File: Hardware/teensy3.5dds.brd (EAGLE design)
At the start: 95.8 x 84.1 mm, 97 parts, among them IC1 AD8034, IC2 AD8034, IC3 AD8034, IC5 AD8034, IC6 AD737KRZ-R7, IC7 AD8034, IC8 AD8034, J1 1776275-2, J2 1776275-2, Q1 10MHz, U1 TEENSY_3.5/3.6_BASIC, U2 ATMEGA32U4-AU, X1 1-227161-0

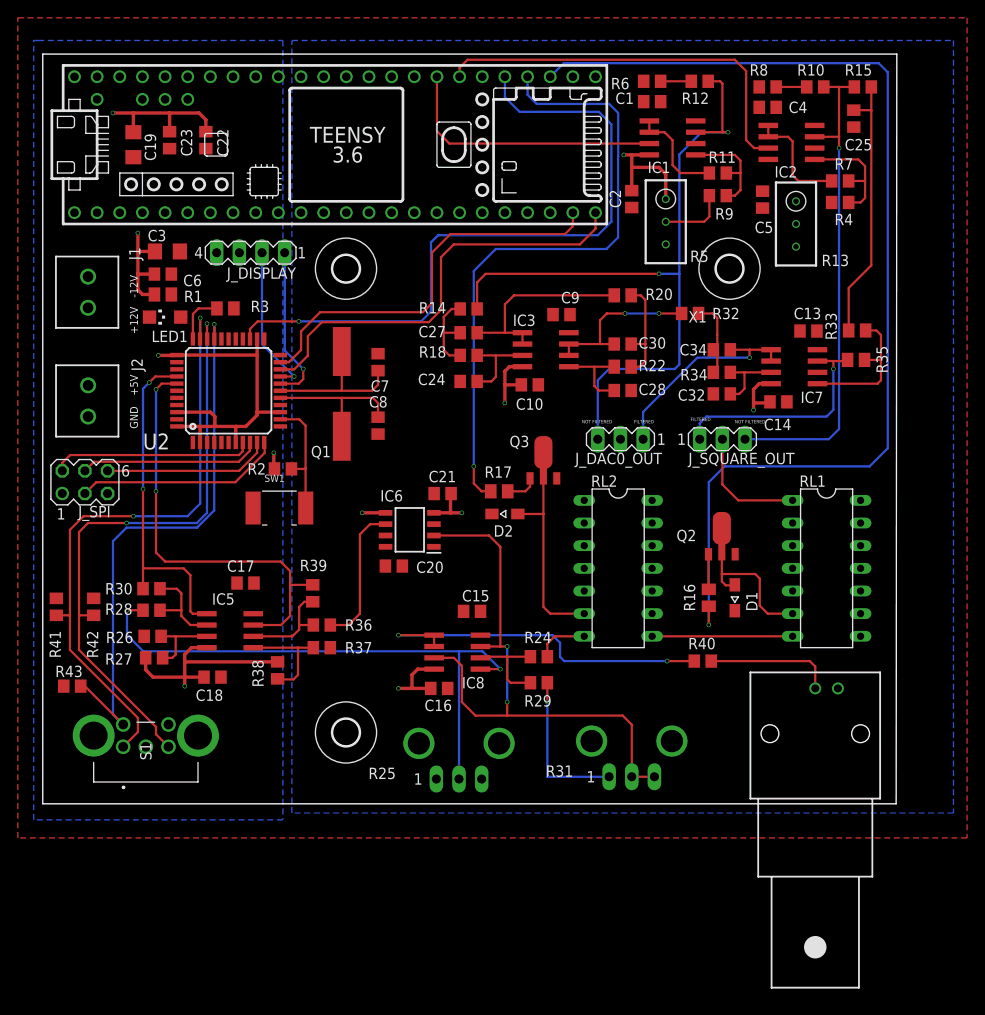
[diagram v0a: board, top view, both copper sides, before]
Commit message: fixes following the advice of people better than me at making PCBs
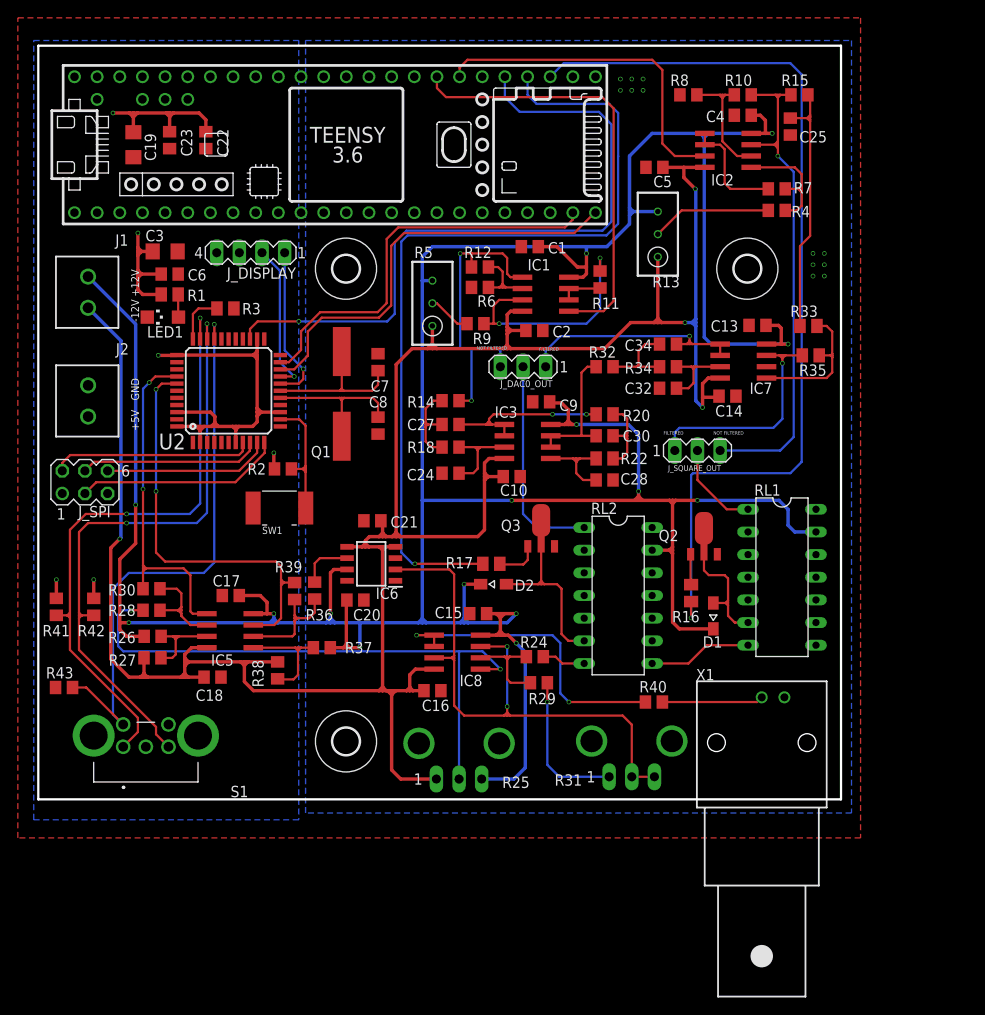
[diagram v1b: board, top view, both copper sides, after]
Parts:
- moved R12 32.3 mm to (49.0, 75.2), turned to 0 degrees
- moved R9 30.7 mm to (48.5, 68.8)
- moved R6 30.1 mm to (49.0, 72.9)
- moved R5 27.7 mm to (43.7, 71.1), turned to 0 degrees
- moved IC1 22.6 mm to (56.4, 72.1)
- moved C1 21.3 mm to (54.6, 77.5)
- moved C2 18.3 mm to (55.1, 68.1), turned to 180 degrees
- moved R11 17.8 mm to (62.5, 73.8), turned to 90 degrees
- moved R13 15.5 mm to (69.0, 78.9), turned to 0 degrees
- moved J_DAC0_OUT 13.6 mm to (53.8, 64.0)
- moved R20 13.5 mm to (63.0, 58.7)
- moved C5 12.7 mm to (68.6, 86.4), turned to 0 degrees
- moved R32 11.3 mm to (63.0, 64.0)
- moved R18 10.5 mm to (45.7, 55.0)
- moved C10 10.5 mm to (52.6, 51.7)
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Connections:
- removed net V-1: R13.1
- net DAC0: now also IC1.5; no longer IC1.3
- net DAC0_OFFSET: now also IC1.1; no longer IC1.7
- net N$21: now also IC1.2; no longer IC1.6
- net N$23: now also IC1.6, IC1.7; no longer IC1.1, IC1.2
- net N$26: now also IC1.3; no longer IC1.5
- net V-: now also R13.1
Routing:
- net V+: track 0.00 -> 409.1 mm, vias 0 -> 15
- net V-: track 68.7 -> 294.1 mm, vias 7 -> 4
- net DAC0_OFFSET: track 83.6 -> 35.0 mm
- net DAC0_SEL: track 70.8 -> 95.1 mm
- net DAC0_OUT: track 0.00 -> 24.0 mm
- net DAC0: track 30.5 -> 49.1 mm
- net SQUARE_SEL: track 120.8 -> 103.6 mm
- net +5V: track 71.3 -> 87.8 mm, vias 4 -> 6
- net N$26: track 12.0 -> 26.5 mm, vias 0 -> 2
- net N$20: track 0.00 -> 13.5 mm
- net N$24: track 3.43 -> 14.9 mm
- net N$14: track 16.1 -> 5.98 mm
- net N$23: track 11.5 -> 4.79 mm
- net SQUARE: track 44.6 -> 38.2 mm
- net N$19: track 40.6 -> 35.3 mm
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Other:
- board size 95.8 x 84.1 mm -> 90 x 84.5 mm

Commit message: board v1.0
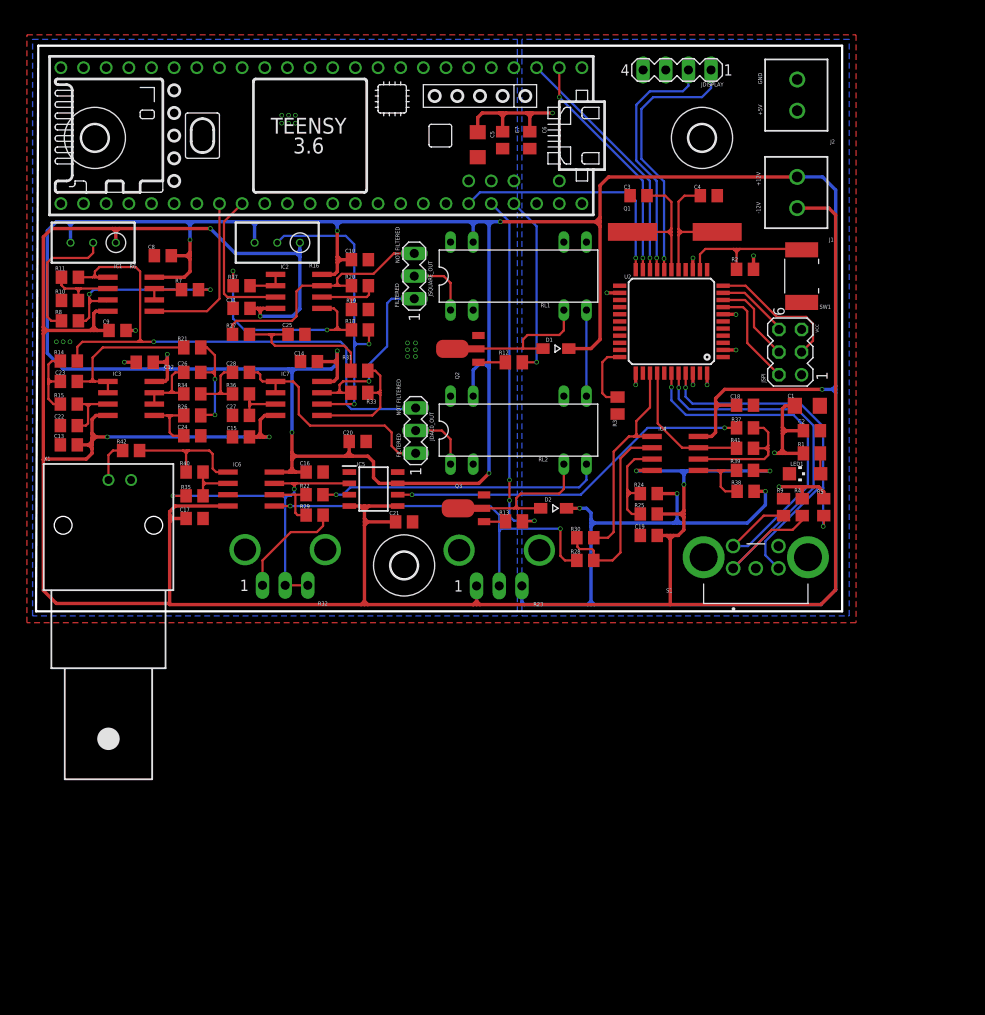
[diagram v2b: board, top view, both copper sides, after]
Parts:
- removed C30, C34: 100p, rcl:C0805
- removed C32: 10p, rcl:C0805
- removed IC8: AD8034, linear:SO08
- removed J_DAC0_OUT, J_SQUARE_OUT: (no value), con-lstb:MA03-1
- removed J_DISPLAY: (no value), con-lstb:MA04-1
- removed J_SPI: (no value), con-lstb:MA03-2
- removed R43: (no value), rcl:R0805
- removed U$5: (no value), holes:3,0
- added C11, C12: 100n, rcl:C0805
- added C26: 100p, rcl:C0805
- added IC4: AD8034, linear:SO08
- added JDAC0_OUT, JSQUARE_OUT: (no value), con-lstb:MA03-1
- added JDISPLAY: (no value), con-lstb:MA04-1
- added JSPI: (no value), con-lstb:MA03-2
- added R19: 1k, rcl:R0805
- added R21: 787, rcl:M0805
- added R23: 10k, Potentiometer_vertical:MA03-1
- added U$1: (no value), holes:3,0
- C1: value 100n -> 1u; device rcl:C0805 -> rcl:C1206
- C19: device rcl:C1206 -> rcl:C0805
- C22: value 100n -> 10p
- C23: value 1u -> 150p
- C25: value (none) -> 1p
- C27: value 100p -> 10p
- C28: value 10p -> 100p
- C3: value 1u -> 22p; device rcl:C1206 -> rcl:C0805
- C4: value 100n -> 22p
- C5: device rcl:C0805 -> rcl:C1206
- C7: value 22p -> 1u
- C8: value 22p -> 100n
- IC5: value AD8034 -> AD737KRZ-R7; device linear:SO08 -> AD737KRZ-R7:SOIC127P600X175-8N
- IC6: value AD737KRZ-R7 -> AD8034; device AD737KRZ-R7:SOIC127P600X175-8N -> linear:SO08
- Q1: value 10MHz -> 16MHz
- R12: value 1k -> 500; device rcl:R0805 -> rcl:M0805
- R13: value 100k -> 500; device rcl:RTRIM3296W -> rcl:M0805
- R15: value (none) -> 2.74k
- R16: value (none) -> 100k; device rcl:M0805 -> rcl:RTRIM3296W
- R17: value (none) -> 1k; device rcl:M0805 -> rcl:R0805
- R18: value 2.74k -> 1k
- R20: value 787 -> 1k; device rcl:M0805 -> rcl:R0805
- R22: value 14.3k -> 1k; device rcl:M0805 -> rcl:R0805
- R25: value 10k -> 1.5k; device Potentiometer_vertical:MA03-1 -> rcl:R0805
- R26: value (none) -> 14.3k; device rcl:R0805 -> rcl:M0805
- R27, R42: value (none) -> 50
- R28, R37: value (none) -> 5k
- R30, R41: value (none) -> 1k
- R31: value 10k -> 2k; device Potentiometer_vertical:MA03-1 -> rcl:M0805
- R32: value 562 -> 10k; device rcl:R0805 -> Potentiometer_vertical:MA03-1
- R33: value 243 -> 10k
- R34: value 20k -> 562
- R35: value 1.78k -> (none); device rcl:M0805 -> rcl:R0805
- R36: value (none) -> 20k
- R38: value (none) -> 10k
- R39: value (none) -> 14.3k
- R4, R9: value 1k -> 10k
- R40: value 50 -> (none)
- R5: value 100k -> 10k; device rcl:RTRIM3296W -> rcl:R0805
- R6: value 1k -> 100k; device rcl:R0805 -> rcl:RTRIM3296W
- RL1, RL2: value PRME_15005SOCKET -> PRME_15005NOSOCKET; device prme15005:DIL14_SOCKET -> prme15005:DIL14
- moved R15 89.0 mm to (2.92, 59.8), turned to 0 degrees
- moved J2 86.6 mm to (84.6, 92.7)
- moved J1 80.3 mm to (84.6, 81.8)
- moved R41 79.2 mm to (78.7, 54.9), turned to 180 degrees
- moved R10 78.9 mm to (3.05, 71.4)
- moved C13 78.4 mm to (2.92, 55.2), turned to 0 degrees
- moved X1 77.2 mm to (7.37, 46.2)
- moved R1 74.2 mm to (86.2, 54.3)
- moved LED1 74.1 mm to (85.5, 52.0)
- moved R8 73.8 mm to (3.05, 69.2), turned to 0 degrees
- moved C19 72.5 mm to (67.9, 45.1), turned to 0 degrees
- moved S1 71.3 mm to (79.9, 40.4)
- moved R35 70.9 mm to (17.0, 49.5), turned to 0 degrees
- moved C18 67.0 mm to (78.7, 59.7), turned to 0 degrees
- moved R7 66.7 mm to (16.5, 72.6)
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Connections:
- removed net N$20: R13.2, R4.1
- new net N$36: IC6.2, R35.2, R40.1
- new net N$37: IC7.6, R16.2, R18.1
- net +5V: now also C1.1, C2.1, C5.1, C7.1, JDISPLAY.3, JSPI.5, R4.1, R5.1; no longer C19.1, C22.1, C23.1, C3.1, J_DISPLAY.3, J_SPI.5, R41.1, R42.1
- net AMPL_MEASURE: now also IC4.7, R41.2, U2.37; no longer IC5.7, R39.2, U2.38
- net DAC0_FILTERED: now also C28.1, JDAC0_OUT.1; no longer C34.1, J_DAC0_OUT.1
- net DAC0_OFFSET: now also JDAC0_OUT.3, R11.1; no longer J_DAC0_OUT.3, R12.1
- net DAC0_OUT: now also JDAC0_OUT.2; no longer J_DAC0_OUT.2
- net DAC0_SEL: now also R13.1, U1.22/A8; no longer R17.1, U1.36/A17
- net GND: now also C10.2, C11.1, C12.2, C13.1, C14.2, C15.1, C16.2, C17.1, C18.2, C19.1, C2.2, C22.1, C27.1, C3.1, C4.1, C5.2, C7.2, C8.2, C9.1, IC5.3, IC5.8, JDISPLAY.4, JSPI.1, R10.2, R19.2, R9.1; no longer C10.1, C13.2, C14.1, C15.2, C16.1, C17.2, C18.1, C19.2, C2.1, C22.2, C23.2, C28.1, C3.2, C32.1, C4.2, C5.1, C7.1, C8.1, C9.2, IC6.8, IC7.6, J_DISPLAY.4, J_SPI.1, R43.1, R6.2, R8.2
- net INTERRUPT: now also U1.21/A7, U2.22; no longer U1.37/A18, U2.25
- net MISO: now also JSPI.3; no longer J_SPI.3
- net MOSI: now also JSPI.6; no longer J_SPI.6
- net N$1: now also R31.2, R33.1; no longer R33.2, R35.1
- net N$10: now also R22.1; no longer R24.1
- net N$11: now also IC4.2; no longer IC5.2
- net N$13: now also IC4.3, R24.1, R25.2; no longer IC5.3, R26.1, R27.2
- net N$14: now also IC5.6, R37.1; no longer IC6.6, R36.1
- net N$15: now also R32.1; no longer R31.1
- net N$16: now also IC4.6, R37.2, R41.1; no longer IC5.6, R36.2, R39.1
- net N$17: now also R12.2; no longer R16.2
- net N$18: now also R13.2; no longer R17.2
- net N$19: now also IC6.1, R40.2, R42.1; no longer IC8.1, IC8.2, R40.1
- net N$21: now also R10.1, R11.2; no longer R12.2, R6.1
- net N$22: now also IC4.5, R38.2, R39.1; no longer IC5.5, R37.2, R38.1
- net N$23: now also R7.1; no longer R11.1
- net N$24: now also R19.1, R20.2; no longer R10.2, R8.1
- net N$25: now also R4.2, U2.40; no longer R41.2, U2.32
- net N$26: now also R7.2, R8.2; no longer R11.2, R9.2
- net N$27: now also R17.1; no longer R7.1
- net N$28: now also R17.2, R18.2; no longer R4.2, R7.2
- net N$29: now also R9.2, U2.39; no longer R43.2, U2.30
- net N$3: now also IC6.5, R23.2; no longer IC8.5, R25.2
- net N$31: now also C3.2; no longer C7.2
- net N$34: now also R27.1, R31.1; no longer R15.1, R33.1
- net N$4: now also C4.2; no longer C8.2
- net N$5: now also IC6.6, R22.2; no longer IC8.6, R24.2
- net N$50: now also C23.2, R15.1; no longer C27.2, R18.1
- net N$53: now also C23.1, R21.1; no longer C27.1, R20.1
- net N$56: now also R6.2, R8.1; no longer R5.2, R9.1
- net N$58: now also C22.2, R15.2; no longer C24.2, R18.2
- net N$6: now also R42.2; no longer R40.2
- net N$61: now also C26.1, R21.2, R26.1; no longer C30.1, R20.2, R22.1
- net N$62: now also C26.2, R34.1; no longer C30.2, R32.1
- net N$63: now also C24.2, R26.2; no longer C28.2, R22.2
- net N$73: now also C28.2, R34.2, R36.1; no longer C34.2, R32.2, R34.1
- net N$75: now also C27.2, R36.2; no longer C32.2, R34.2
- net N$8: now also R5.2, U2.41; no longer R42.2, U2.31
- net N$9: now also IC5.2, IC6.7, R32.2, R32.3, R35.1; no longer IC6.2, IC8.3, IC8.7, R31.2, R31.3
- net OFF_MEASURE: now also IC4.1, U2.36; no longer IC5.1, U2.37
- net RX1: now also U1.1/TX; no longer U1.32/A13
- net SCK: now also JSPI.4; no longer J_SPI.4
- net SCL: now also JDISPLAY.1; no longer J_DISPLAY.1
- net SDA: now also JDISPLAY.2; no longer J_DISPLAY.2
- net SQUARE: now also U1.A22/DAC1; no longer U1.39/A20
- net SQUARE_FILTERED: now also JSQUARE_OUT.1, R33.2; no longer J_SQUARE_OUT.1, R35.2
- net SQUARE_OFFSET: now also JSQUARE_OUT.3, R20.1, R27.2; no longer J_SQUARE_OUT.3, R10.1, R15.2
- net SQUARE_OUT: now also JSQUARE_OUT.2; no longer J_SQUARE_OUT.2
- net SQUARE_SEL: now also R12.1, U1.23/A9; no longer R16.1, U1.35/A16
- net SS: now also JSPI.2; no longer J_SPI.2
- net TX1: now also U1.0/RX; no longer U1.31/A12
- net V+: now also C10.1, C12.1, C14.1, C16.1, C18.1, C8.1, IC4.8, IC5.7, IC6.8, R16.3, R23.3, R24.2, R38.1, R6.3; no longer C1.1, C13.1, C15.1, C17.1, C4.1, C9.1, IC5.8, IC6.7, IC8.8, R13.3, R25.3, R26.2, R37.1, R5.3
- net V-: now also C11.2, C13.2, C15.2, C17.2, C19.2, C9.2, IC4.4, IC5.5, R16.1, R23.1, R39.2, R6.1; no longer C10.2, C14.2, C16.2, C18.2, C2.2, C5.2, IC6.5, IC8.4, R13.1, R27.1, R38.2, R5.1
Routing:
- net SQUARE_SEL: track 103.6 -> 20.4 mm
- net V-: track 294.1 -> 372.0 mm, vias 4 -> 7
- net DAC0_SEL: track 95.1 -> 40.3 mm, vias 1 -> 3
- net INTERRUPT: track 77.7 -> 27.4 mm
- net V+: track 409.1 -> 447.7 mm, vias 15 -> 11
- net +5V: track 87.8 -> 50.2 mm, vias 6 -> 11
- net N$14: track 5.98 -> 41.1 mm, vias 0 -> 2
- net N$37: track 0.00 -> 34.9 mm, vias 0 -> 2
- net AMPL_MEASURE: track 47.2 -> 15.7 mm, vias 2 -> 0
- net DAC0: track 49.1 -> 18.6 mm
- net DAC0_OFFSET: track 35.0 -> 65.4 mm, vias 2 -> 1
- net SQUARE_OFFSET: track 58.6 -> 29.2 mm, vias 1 -> 0
- net N$9: track 65.4 -> 39.0 mm
- net N$10: track 16.5 -> 41.7 mm, vias 0 -> 1
- net N$8: track 68.9 -> 44.5 mm
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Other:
- board size 90 x 84.5 mm -> 90.4 x 63.4 mm
- board text added: "vcc"
